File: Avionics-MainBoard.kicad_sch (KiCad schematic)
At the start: 4 parts

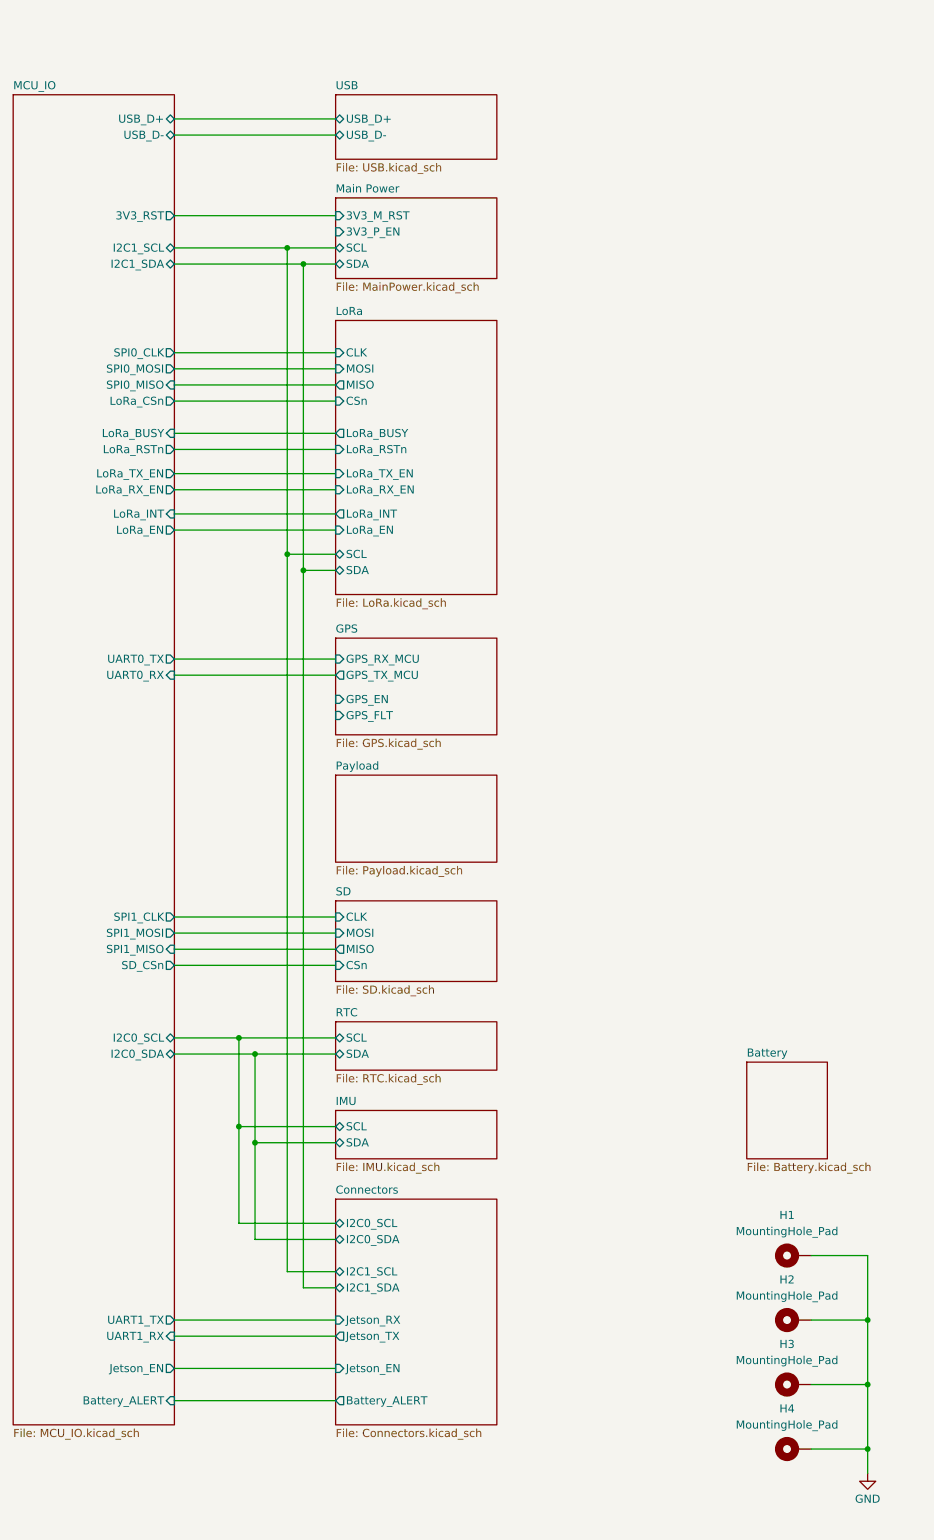
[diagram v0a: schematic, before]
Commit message: v3 Layout complete
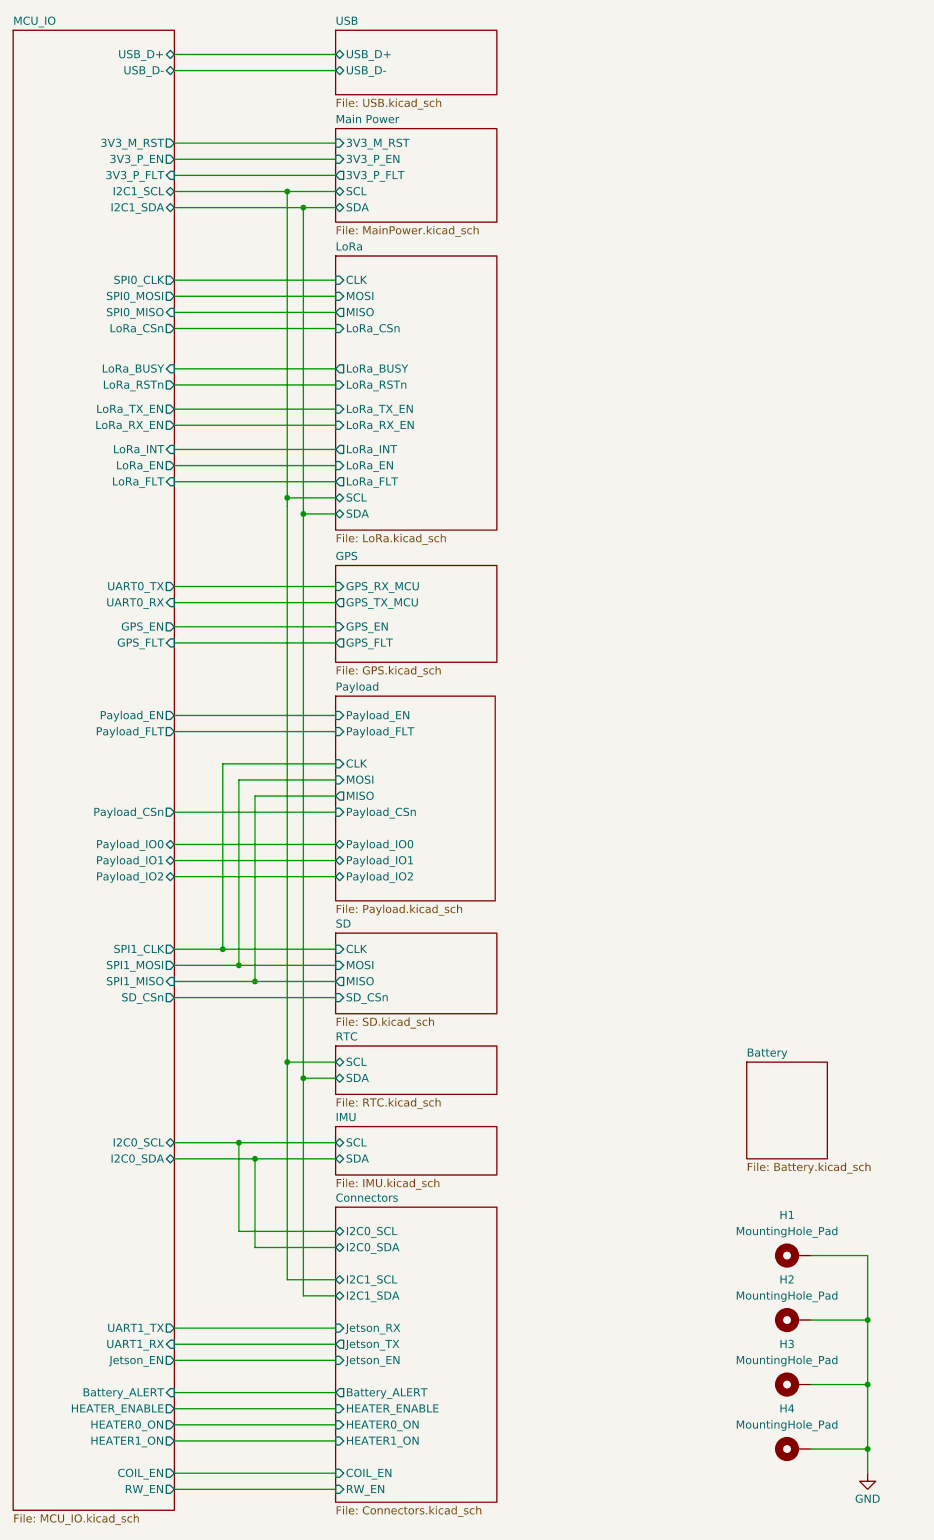
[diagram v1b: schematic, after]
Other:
- sheet Connectors ports: added COIL_EN, HEATER0_ON, HEATER1_ON, HEATER_ENABLE, RW_EN; removed none
- sheet LoRa ports: added LoRa_CSn, LoRa_FLT; removed CSn
- sheet MCU_IO ports: added 3V3_M_RST, 3V3_P_EN, 3V3_P_FLT, COIL_EN, GPS_EN, GPS_FLT, HEATER0_ON, HEATER1_ON, HEATER_ENABLE, LoRa_FLT, Payload_CSn, Payload_EN, Payload_FLT, Payload_IO0, Payload_IO1, Payload_IO2, RW_EN; removed 3V3_RST
- sheet Main Power ports: added 3V3_P_FLT; removed none
- sheet Payload ports: added CLK, MISO, MOSI, Payload_CSn, Payload_EN, Payload_FLT, Payload_IO0, Payload_IO1, Payload_IO2; removed none
- sheet SD ports: added SD_CSn; removed CSn
